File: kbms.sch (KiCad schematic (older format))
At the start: 13 parts, among them J12 AVR-ISP-6, J13 DE9 Male, J14 DE9 Male, J15 Mini-DIN-6, J16 Mini-DIN-6, U6 ATmega328-PU

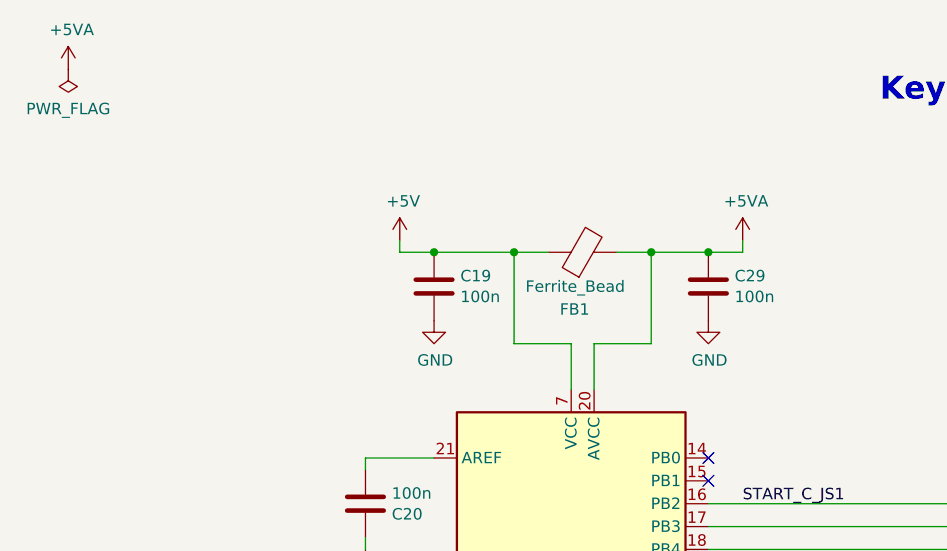
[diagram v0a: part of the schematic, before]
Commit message: Work in progress.
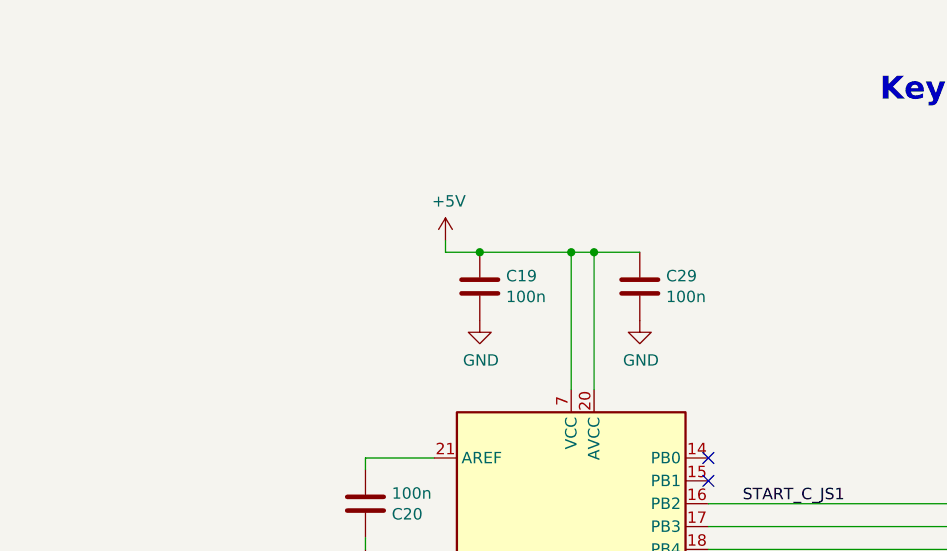
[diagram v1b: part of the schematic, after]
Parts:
- removed FB1: Ferrite_Bead, Inductor_THT:L_Axial_L12.8mm_D5.8mm_P5.08mm_Vertical_Fastron_HBCC, symbol Device:Ferrite_Bead
- J12: footprint (none) -> Connector_PinHeader_2.54mm:PinHeader_2x03_P2.54mm_Vertical
- R19, R20, R21: footprint (none) -> Resistor_THT:R_Axial_DIN0411_L9.9mm_D3.6mm_P12.70mm_Horizontal
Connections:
- net labels removed: +5VA
- wire segments 106 -> 99
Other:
- moved on the sheet: C19, C29
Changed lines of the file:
@@
 L power:+5V #PWR?
 U 1 1 5E1A9904
-P 2350 1650
+P 2550 1650
 AR Path="/5E1A9904" Ref="#PWR?"  Part="1"
 AR Path="/5DF2662E/5E1A9904" Ref="#PWR047"  Part="1"
-F 0 "#PWR047" H 2350 1500 50  0001 C CNN
-F 1 "+5V" H 2365 1823 50  0000 C CNN
-F 2 "" H 2350 1650 50  0001 C CNN
-F 3 "" H 2350 1650 50  0001 C CNN
-	1    2350 1650
+F 0 "#PWR047" H 2550 1500 50  0001 C CNN
+F 1 "+5V" H 2565 1823 50  0000 C CNN
+F 2 "" H 2550 1650 50  0001 C CNN
+F 3 "" H 2550 1650 50  0001 C CNN
+	1    2550 1650
 	1    0    0    -1
 $EndComp
@@
 F 0 "R19" V 5300 3050 50  0000 C CNN
 F 1 "1k" V 5300 3400 50  0000 C CNN
-F 2 "" V 5180 3250 50  0001 C CNN
+F 2 "Resistor_THT:R_Axial_DIN0411_L9.9mm_D3.6mm_P12.70mm_Horizontal" V 5180 3250 50  0001 C CNN
 F 3 "~" H 5250 3250 50  0001 C CNN
 	1    5250 3250
@@
 F 0 "R20" V 5300 3200 50  0000 C CNN
 F 1 "1k" V 5300 3550 50  0000 C CNN
-F 2 "" V 5180 3400 50  0001 C CNN
+F 2 "Resistor_THT:R_Axial_DIN0411_L9.9mm_D3.6mm_P12.70mm_Horizontal" V 5180 3400 50  0001 C CNN
 F 3 "~" H 5250 3400 50  0001 C CNN
 	1    5250 3400
@@
 F 0 "R21" V 5300 3350 50  0000 C CNN
 F 1 "1k" V 5300 3700 50  0000 C CNN
-F 2 "" V 5180 3550 50  0001 C CNN
+F 2 "Resistor_THT:R_Axial_DIN0411_L9.9mm_D3.6mm_P12.70mm_Horizontal" V 5180 3550 50  0001 C CNN
 F 3 "~" H 5250 3550 50  0001 C CNN
 	1    5250 3550
 	0    1    1    0
 $EndComp
-$Comp
-L Device:Ferrite_Bead FB1
-U 1 1 5E23A02B
-P 3150 1700
-F 0 "FB1" V 2900 1800 50  0000 R CNN
-F 1 "Ferrite_Bead" V 3000 1950 50  0000 R CNN
-F 2 "Inductor_THT:L_Axial_L12.8mm_D5.8mm_P5.08mm_Vertical_Fastron_HBCC" V 3080 1700 50  0001 C CNN
-F 3 "https://abracon.com/Magnetics/chokes/AWBC-09.pdf" H 3150 1700 50  0001 C CNN
-F 4 "535-12742-ND" V 3150 1700 50  0001 C CNN "Digikey"
-	1    3150 1700
-	0    -1   -1   0
-$EndComp
-Wire Wire Line
-	2350 1650 2350 1700
+Wire Wire Line
+	2550 1650 2550 1700
 $Comp
 L Device:C C?
 U 1 1 5DF43DC7
-P 2500 1850
+P 2700 1850
 AR Path="/5DF43DC7" Ref="C?"  Part="1"
 AR Path="/5DF2662E/5DF43DC7" Ref="C19"  Part="1"
-F 0 "C19" H 2615 1896 50  0000 L CNN
-F 1 "100n" H 2615 1805 50  0000 L CNN
-F 2 "Capacitor_THT:C_Disc_D3.0mm_W2.0mm_P2.50mm" H 2538 1700 50  0001 C CNN
-F 3 "~" H 2500 1850 50  0001 C CNN
-	1    2500 1850
+F 0 "C19" H 2815 1896 50  0000 L CNN
+F 1 "100n" H 2815 1805 50  0000 L CNN
+F 2 "Capacitor_THT:C_Disc_D3.0mm_W2.0mm_P2.50mm" H 2738 1700 50  0001 C CNN
+F 3 "~" H 2700 1850 50  0001 C CNN
+	1    2700 1850
 	1    0    0    -1
 $EndComp
@@
 L power:GND #PWR?
 U 1 1 5DF43DD3
-P 2500 2000
+P 2700 2000
 AR Path="/5DF43DD3" Ref="#PWR?"  Part="1"
 AR Path="/5DF2662E/5DF43DD3" Ref="#PWR045"  Part="1"
-F 0 "#PWR045" H 2500 1750 50  0001 C CNN
-F 1 "GND" H 2505 1827 50  0000 C CNN
-F 2 "" H 2500 2000 50  0001 C CNN
-F 3 "" H 2500 2000 50  0001 C CNN
-	1    2500 2000
+F 0 "#PWR045" H 2700 1750 50  0001 C CNN
+F 1 "GND" H 2705 1827 50  0000 C CNN
+F 2 "" H 2700 2000 50  0001 C CNN
+F 3 "" H 2700 2000 50  0001 C CNN
+	1    2700 2000
 	1    0    0    -1
 $EndComp
@@
 F 0 "J12" H 6520 2346 50  0000 R CNN
 F 1 "AVR-ISP-6" H 6520 2255 50  0000 R CNN
-F 2 "" V 6600 2300 50  0001 C CNN
+F 2 "Connector_PinHeader_2.54mm:PinHeader_2x03_P2.54mm_Vertical" V 6600 2300 50  0001 C CNN
 F 3 " ~" H 5575 1700 50  0001 C CNN
 	1    6850 2250
@@
 L Device:C C?
 U 1 1 5E043F05
-P 3700 1850
+P 3400 1850
 AR Path="/5E043F05" Ref="C?"  Part="1"
 AR Path="/5DF2662E/5E043F05" Ref="C29"  Part="1"
-F 0 "C29" H 3815 1896 50  0000 L CNN
-F 1 "100n" H 3815 1805 50  0000 L CNN
-F 2 "Capacitor_THT:C_Disc_D3.0mm_W2.0mm_P2.50mm" H 3738 1700 50  0001 C CNN
-F 3 "~" H 3700 1850 50  0001 C CNN
-	1    3700 1850
+F 0 "C29" H 3515 1896 50  0000 L CNN
+F 1 "100n" H 3515 1805 50  0000 L CNN
+F 2 "Capacitor_THT:C_Disc_D3.0mm_W2.0mm_P2.50mm" H 3438 1700 50  0001 C CNN
+F 3 "~" H 3400 1850 50  0001 C CNN
+	1    3400 1850
 	1    0    0    -1
 $EndComp
@@
 L power:GND #PWR?
 U 1 1 5E044959
-P 3700 2000
+P 3400 2000
 AR Path="/5E044959" Ref="#PWR?"  Part="1"
 AR Path="/5DF2662E/5E044959" Ref="#PWR044"  Part="1"
-F 0 "#PWR044" H 3700 1750 50  0001 C CNN
-F 1 "GND" H 3705 1827 50  0000 C CNN
-F 2 "" H 3700 2000 50  0001 C CNN
-F 3 "" H 3700 2000 50  0001 C CNN
-	1    3700 2000
-	1    0    0    -1
-$EndComp
-Wire Wire Line
-	3100 2300 3100 2100
-Wire Wire Line
-	3200 2100 3450 2100
-Wire Wire Line
-	3450 2100 3450 1700
-Wire Wire Line
-	3300 1700 3450 1700
-Connection ~ 3450 1700
-Wire Wire Line
-	3450 1700 3700 1700
-Wire Wire Line
-	2500 1700 2350 1700
-Connection ~ 2500 1700
-Wire Wire Line
-	2850 2100 2850 1700
-Wire Wire Line
-	2850 2100 3100 2100
-Wire Wire Line
-	2500 1700 2850 1700
-Connection ~ 2850 1700
-Wire Wire Line
-	2850 1700 3000 1700
-$Comp
-L power:+5VA #PWR0101
-U 1 1 5E068477
-P 3850 1650
-F 0 "#PWR0101" H 3850 1500 50  0001 C CNN
-F 1 "+5VA" H 3865 1823 50  0000 C CNN
-F 2 "" H 3850 1650 50  0001 C CNN
-F 3 "" H 3850 1650 50  0001 C CNN
-	1    3850 1650
-	1    0    0    -1
-$EndComp
-Wire Wire Line
-	3700 1700 3850 1700
-Wire Wire Line
-	3850 1700 3850 1650
-Connection ~ 3700 1700
-$Comp
-L power:PWR_FLAG #FLG0101
-U 1 1 5E0722FD
-P 900 900
-F 0 "#FLG0101" H 900 975 50  0001 C CNN
-F 1 "PWR_FLAG" H 900 1073 50  0000 C CNN
-F 2 "" H 900 900 50  0001 C CNN
-F 3 "~" H 900 900 50  0001 C CNN
-	1    900  900
-	-1   0    0    1
-$EndComp
+F 0 "#PWR044" H 3400 1750 50  0001 C CNN
+F 1 "GND" H 3405 1827 50  0000 C CNN
+F 2 "" H 3400 2000 50  0001 C CNN
+F 3 "" H 3400 2000 50  0001 C CNN
+	1    3400 2000
+	1    0    0    -1
+$EndComp
+Wire Wire Line
+	2700 1700 2550 1700
 $Comp
 L MCU_Microchip_ATmega:ATmega328-PU U6
@@
 $EndComp
 Wire Wire Line
-	3200 2100 3200 2300
-$Comp
-L power:+5VA #PWR0102
-U 1 1 5E078129
-P 900 900
-F 0 "#PWR0102" H 900 750 50  0001 C CNN
-F 1 "+5VA" H 915 1073 50  0000 C CNN
-F 2 "" H 900 900 50  0001 C CNN
-F 3 "" H 900 900 50  0001 C CNN
-	1    900  900
-	1    0    0    -1
-$EndComp
+	3100 1700 3100 2300
+Wire Wire Line
+	3200 1700 3200 2300
+Wire Wire Line
+	2700 1700 3100 1700
+Connection ~ 2700 1700
+Connection ~ 3100 1700
+Wire Wire Line
+	3100 1700 3200 1700
+Connection ~ 3200 1700
+Wire Wire Line
+	3200 1700 3400 1700
 $EndSCHEMATC
